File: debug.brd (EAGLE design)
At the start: 25 x 100 mm, 24 parts, among them CN1 2X10 HEADER, CN2 MICRO USB B, CN3 14 PIN 2mm, CN4 MICRO USB B, CN5 2X10 HEADER, CN6 31 PIN FPC, U1 USBLC6-2SC6, U2 USBLC6-2SC6, U3 FT231X, U7 FT231X

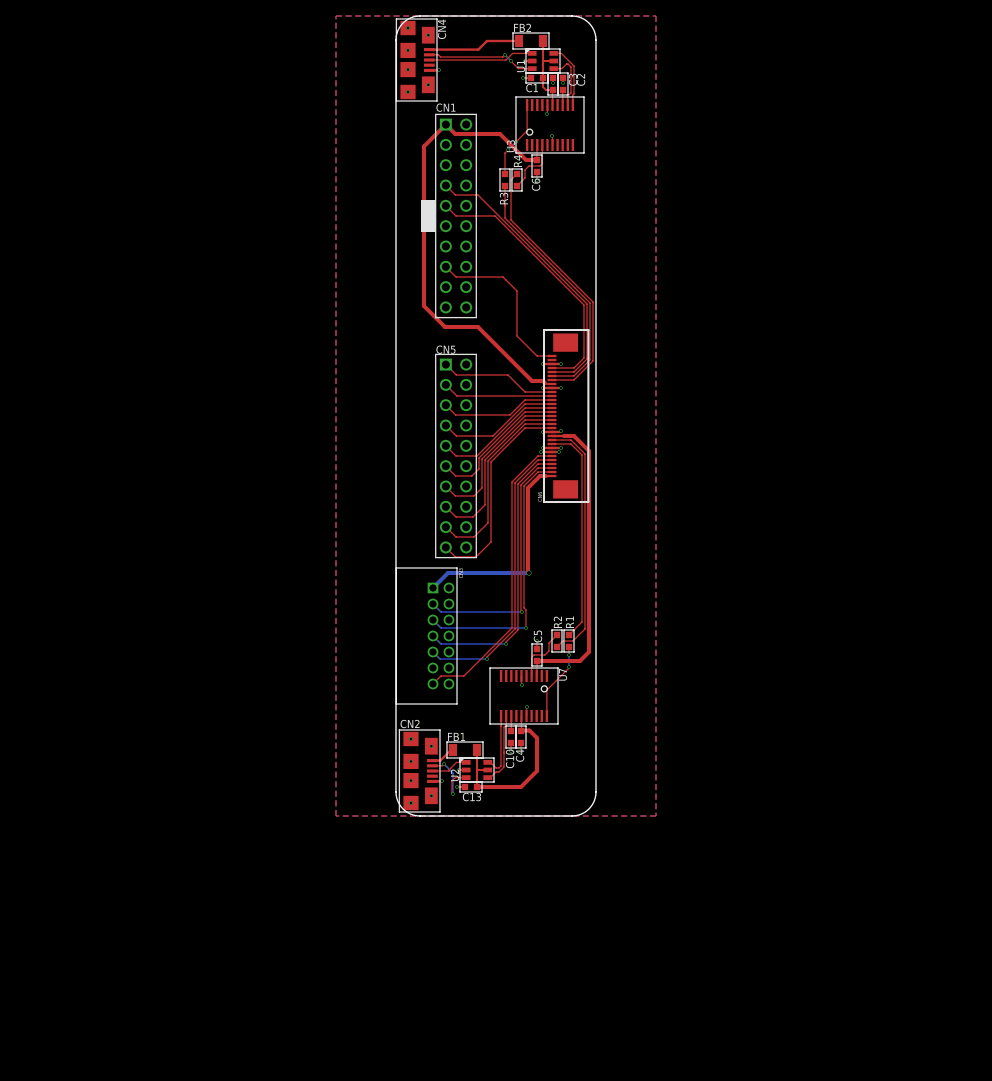
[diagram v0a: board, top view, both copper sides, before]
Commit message: Thumb button connected to wakeup, diff pair lengths fixed
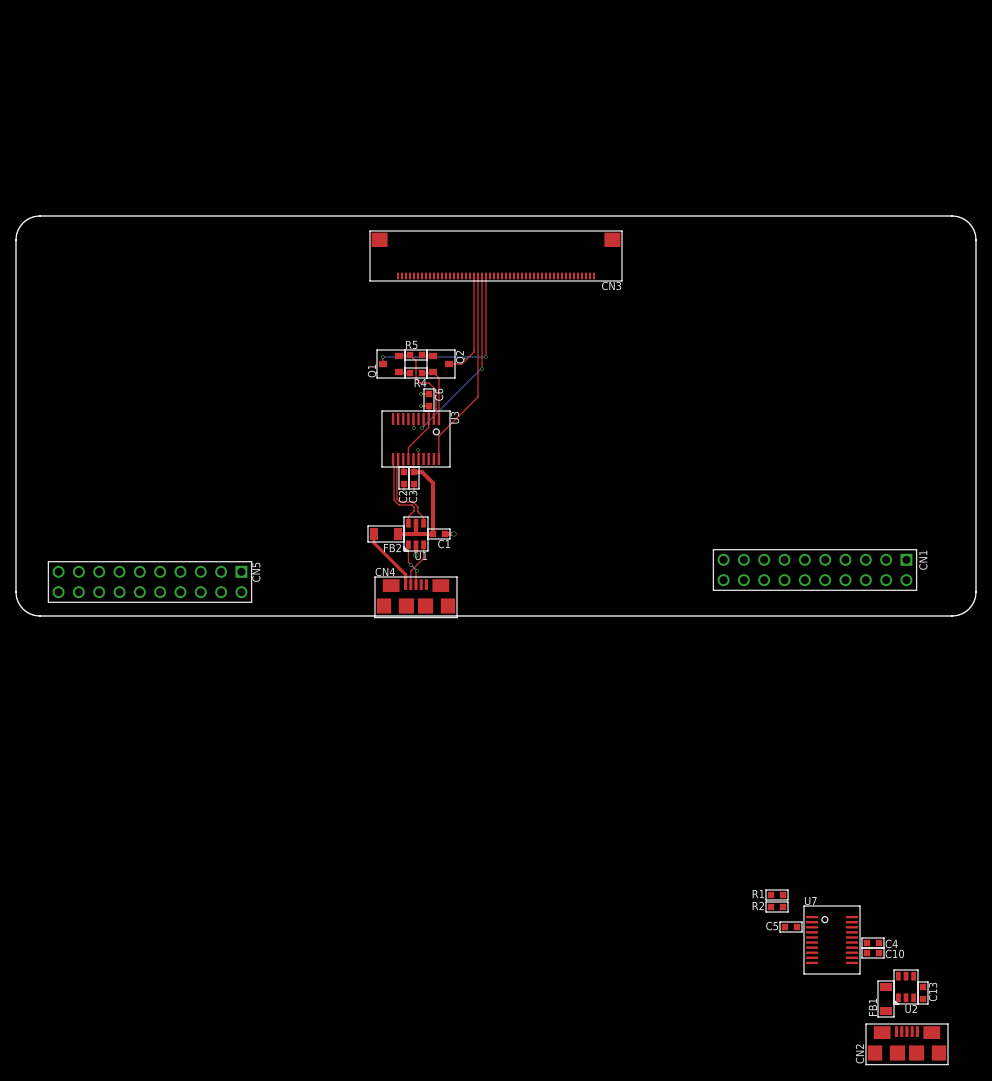
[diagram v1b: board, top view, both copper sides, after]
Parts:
- removed CN6: 31 PIN FPC, CONNECTORs:3-1734839-1
- removed R3: 10R, r_0603:0603
- added Q1, Q2: MMBT3904, TRANSISTORs:SOT23-3
- added R5: 10k, r_0603:0603
- CN3: value 14 PIN 2mm -> 50 PIN 0.5MM; device CONNECTORs:0878331420 -> CONNECTORs:FH52E-50S-0.5SH
- R4: value 10R -> 10k
- moved CN2 71.3 mm to (51.4, -79.6), turned to 0 degrees
- moved CN4 68.3 mm to (-10.0, -23.8), turned to 0 degrees
- moved FB2 64.2 mm to (-13.8, -14.8)
- moved CN1 63.0 mm to (39.9, -19.2), turned to 270 degrees
- moved C13 62.1 mm to (53.4, -72.1), turned to 90 degrees
- moved U1 61.2 mm to (-10.0, -14.8), turned to 180 degrees
- moved FB1 61.1 mm to (48.8, -72.9), turned to 270 degrees
- moved U2 60.1 mm to (51.2, -71.4), turned to 180 degrees
- moved C1 58.3 mm to (-7.12, -14.8), turned to 180 degrees
- moved C2 53.1 mm to (-11.5, -7.75), turned to 90 degrees
- moved C10 52.7 mm to (47.1, -67.1), turned to 180 degrees
- moved C3 52.2 mm to (-10.2, -7.75), turned to 90 degrees
- moved C4 51.0 mm to (47.1, -65.9), turned to 180 degrees
- moved U7 49.1 mm to (42.0, -65.5), turned to 0 degrees
- moved CN3 48.0 mm to (0.00, 20.0), turned to 180 degrees
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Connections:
- net N$13 renamed USB_VBUS
- removed net DEBUG_GPIO_0: CN6.30
- removed net FPGA_JTAG_NRESET: CN3.13, CN6.6
- removed net FPGA_TCK: CN3.5, CN6.2
- removed net FPGA_TDI: CN3.9, CN6.5
- removed net FPGA_TDO: CN3.7, CN6.4
- removed net FPGA_TMS: CN3.3, CN6.3
- removed net N$15: R3.1, U3.20
- removed net N$16: R4.1, U3.4
- removed net STP_UART_RX: CN6.26, R3.2
- removed net STP_UART_TX: CN6.25, R4.2
- new net BMS_I2C_SCL: CN3.P25
- new net BMS_I2C_SDA: CN3.P24
- new net BMS_NINT: CN3.P23
- new net DEBUG_UART_RX: CN3.P34
- new net DEBUG_UART_TX: CN3.P35
- new net ESP32_EN: CN3.P28, Q1.2
- new net ESP32_UART_!DTR: Q2.3, R4.2, U3.1
- new net ESP32_UART_!RTS: Q1.3, R5.2, U3.2
- new net ESP32_UART_RX: CN3.P30, U3.20
- new net ESP32_UART_TX: CN3.P29, U3.4
- new net ESP_IO0: CN3.P31, Q2.2
- new net FPGA_GPIO_0: CN3.P9
- new net FPGA_GPIO_1: CN3.P12
- new net FPGA_GPIO_2: CN3.P14
- new net FPGA_GPIO_3: CN3.P10
- new net FPGA_GPIO_4: CN3.P13
- new net FPGA_GPIO_5: CN3.P11
- new net FPGA_GPIO_6: CN3.P15
- new net FPGA_JTAG_TCK: CN3.P47
- new net FPGA_JTAG_TDI: CN3.P48
- new net FPGA_JTAG_TDO: CN3.P46
- new net FPGA_JTAG_TMS: CN3.P49
- new net N$100: Q2.1, R5.1
- new net N$99: Q1.1, R4.1
- new net PMC_UART_RX: CN3.P3
- new net PMC_UART_TX: CN3.P2
- new net PSS_JTAG_MOD: CN3.P41
- new net PSS_JTAG_NTRST: CN3.P40
- new net PSS_JTAG_TCK: CN3.P42
- new net PSS_JTAG_TDI: CN3.P39
- new net PSS_JTAG_TDO: CN3.P38
- new net PSS_JTAG_TMS: CN3.P43
- new net PWR_DIG_1V8: CN3.P16, CN3.P45
- new net PWR_PSS_DCDC_1V8: CN3.P33, CN3.P37
- new net PWR_SYS_1V8_SLP: CN3.P7
- net FPGA_DEBUG_CLK: no longer CN6.13
- net FPGA_DEBUG_D0: no longer CN6.15
- net FPGA_DEBUG_D1: no longer CN6.16
- net FPGA_DEBUG_D2: no longer CN6.17
- net FPGA_DEBUG_D3: no longer CN6.18
- net FPGA_DEBUG_D4: no longer CN6.19
- net FPGA_DEBUG_D5: no longer CN6.20
- net FPGA_DEBUG_D6: no longer CN6.21
- net FPGA_DEBUG_D7: no longer CN6.22
- net FPGA_DEBUG_EN: no longer CN6.14
- net FPGA_UART_RX: no longer CN6.9
- net FPGA_UART_TX: no longer CN6.10
- net GND: now also CN3.P1, CN3.P17, CN3.P26, CN3.P32, CN3.P36, CN3.P44, CN3.P50, CN3.P8, CN3.SH1, CN3.SH2; no longer CN3.10, CN3.12, CN3.14, CN3.2, CN3.4, CN3.6, CN3.8, CN6.12, CN6.23, CN6.29, CN6.7, CN6.8
- net PWR_3V3_SLP: no longer C6.2, CN6.24, U3.3
- net PWR_FPGA_1V8: no longer CN6.11
- net PWR_SYS_3V3: now also C6.2, CN3.P27, U3.14, U3.3; no longer CN3.1, CN6.1
- net STP_NRESET: now also CN3.P6; no longer CN6.31
- net STP_SWCLK: now also CN3.P5; no longer CN6.28
- net STP_SWDIO: now also CN3.P4; no longer CN6.27
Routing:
- net PWR_3V3_SLP: track 59.0 -> 0.00 mm
- net PWR_FPGA_1V8: track 39.4 -> 0.00 mm
- net FPGA_JTAG_NRESET: track 37.4 -> 0.00 mm
- net FPGA_TDI: track 36.4 -> 0.00 mm, vias 1 -> 0
- net STP_SWDIO: track 35.7 -> 0.00 mm
- net FPGA_TDO: track 35.4 -> 0.00 mm, vias 1 -> 0
- net FPGA_TCK: track 34.1 -> 0.00 mm, vias 1 -> 0
- net STP_UART_TX: track 34.0 -> 0.00 mm
- net STP_SWCLK: track 33.5 -> 0.00 mm
- net FPGA_TMS: track 32.2 -> 0.00 mm, vias 1 -> 0
- net STP_UART_RX: track 31.7 -> 0.00 mm
- net FPGA_UART_TX: track 31.2 -> 0.00 mm
- net FPGA_UART_RX: track 27.5 -> 0.00 mm
- net FPGA_DEBUG_CLK: track 26.3 -> 0.00 mm
- net ESP32_UART_RX: track 0.00 -> 24.9 mm
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- removed copper zone on layer 1, net GND
- removed copper zone on layer 16, net GND
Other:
- board size 25 x 100 mm -> 120 x 50 mm
